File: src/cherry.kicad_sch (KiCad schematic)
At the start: 72 parts, among them J1 USB4085-GF-A, J2 PinHeader_1x24, J3 PinHeader_1x06, J4 PinHeader_1x06, J5 PinHeader_1x06, J6 PinHeader_1x24, SW1 RESET, SW2 USER, U1 FT2232HQ, U2 ICE40LP8K-CM81, U3 W25Q32JVSSIQ, U4 TPS62A02, U5 TPS62A02, X1 ASE-12.000MHZ-LC-T

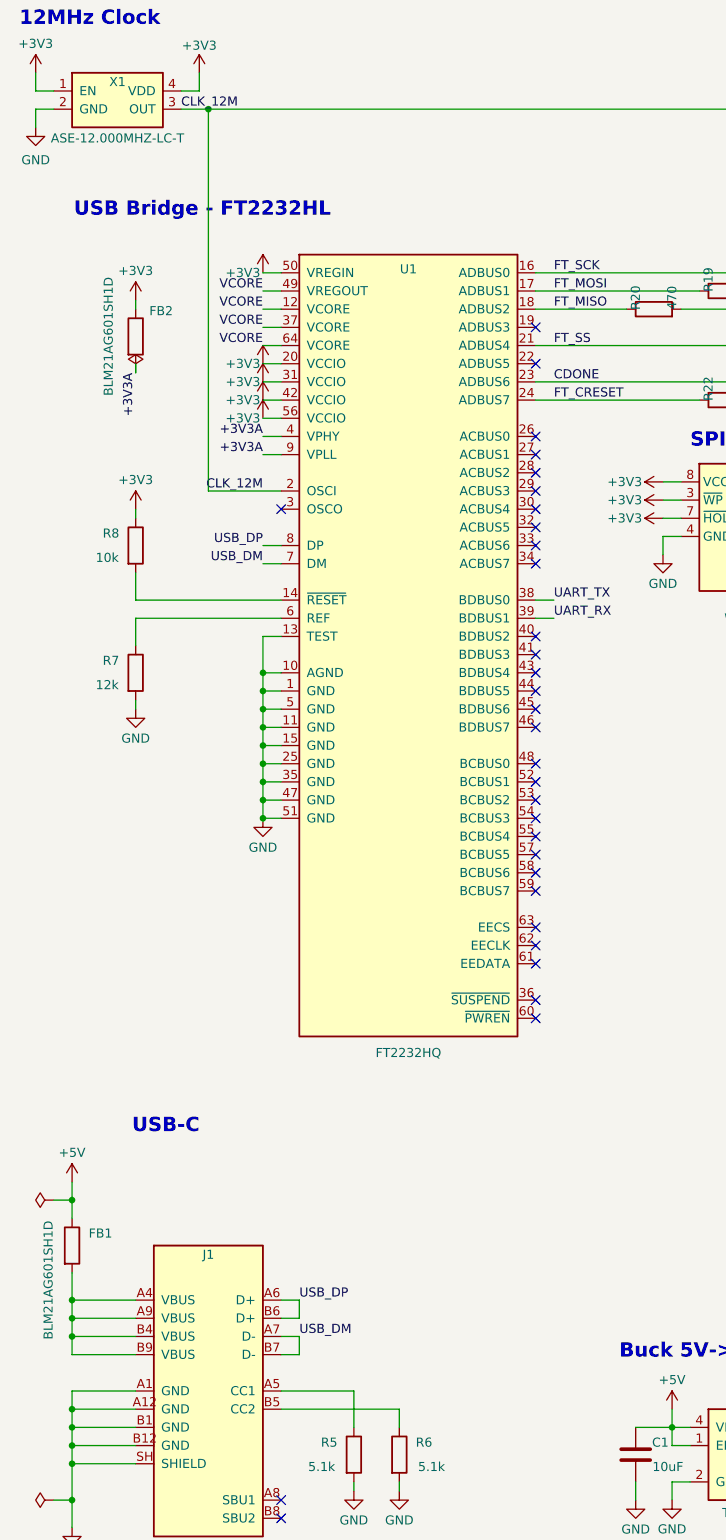
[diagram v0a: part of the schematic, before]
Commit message: 56Q
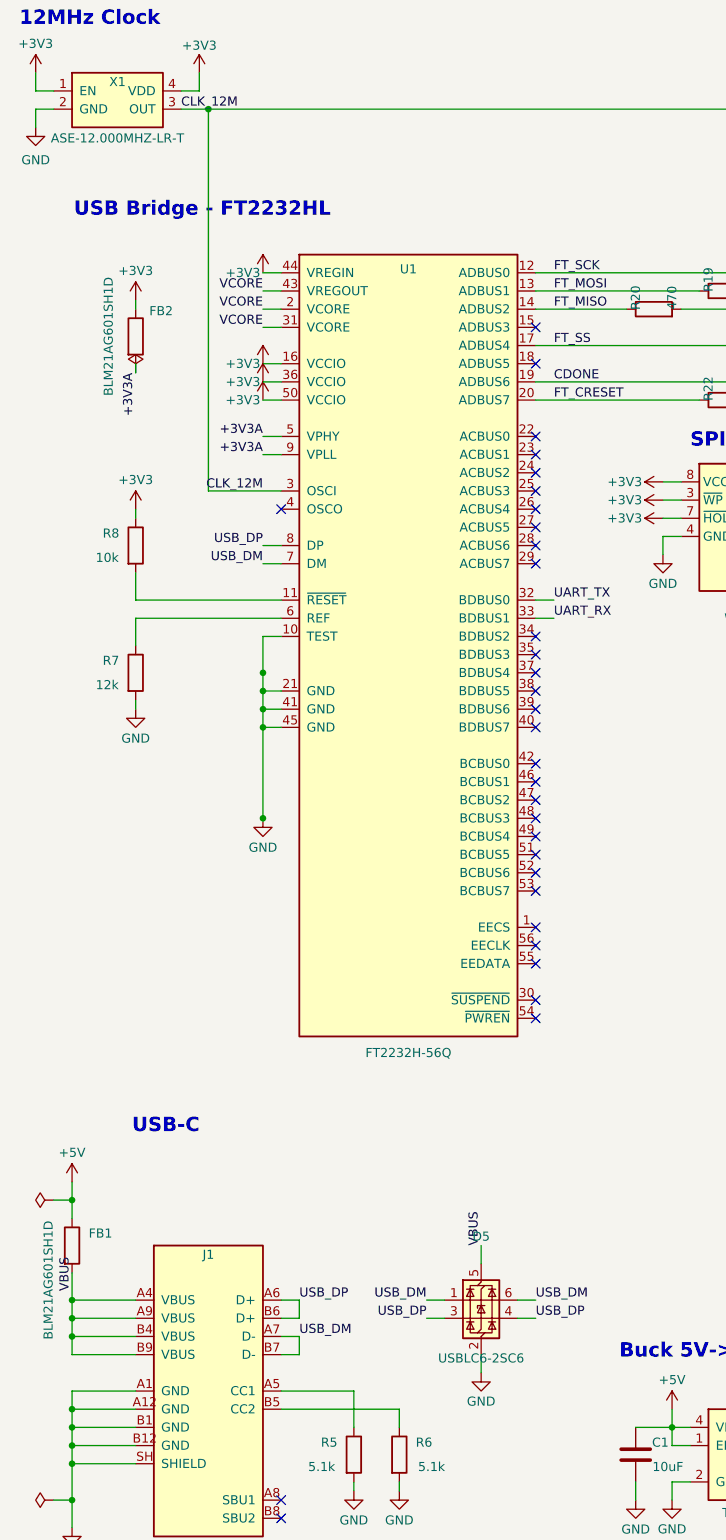
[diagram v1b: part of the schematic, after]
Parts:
- added D5: USBLC6-2SC6, Cherry:SOT-23-6, symbol Cherry:USBLC6-2SC6
- U1: value FT2232HQ -> FT2232H-56Q; footprint Cherry:QFN-64-1EP_9x9mm_P0.5mm_EP4.35x4.35mm -> Cherry:QFN-56-1EP_8x8mm_P0.5mm_EP5.9x5.9mm; symbol Cherry:FT2232HL -> Cherry:FT2232H-56Q
- U3: footprint Cherry:SOIC-8_3.9x4.9mm_P1.27mm -> Cherry:SOIC-8_5.3x5.3mm_P1.27mm
- X1: value ASE-12.000MHZ-LC-T -> ASE-12.000MHZ-LR-T
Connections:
- net +3V3: now also U1.16 (VCCIO), U1.36 (VCCIO), U1.44 (VREGIN); no longer U1.20 (VCCIO), U1.31 (VCCIO), U1.42 (VCCIO), U1.56 (VCCIO)
- net +3V3A: now also U1.5 (VPHY); no longer U1.4 (VPHY)
- net CDONE: now also U1.19 (ADBUS6); no longer U1.23 (ADBUS6)
- net CLK_12M: now also U1.3 (OSCI); no longer U1.2 (OSCI)
- net FT_CRESET: now also U1.20 (ADBUS7); no longer U1.24 (ADBUS7)
- net FT_MISO: now also U1.14 (ADBUS2); no longer U1.18 (ADBUS2)
- net FT_MOSI: now also U1.13 (ADBUS1); no longer U1.17 (ADBUS1)
- net FT_SCK: now also U1.12 (ADBUS0); no longer U1.16 (ADBUS0)
- net FT_SS: now also U1.17 (ADBUS4); no longer U1.21 (ADBUS4)
- net GND: now also U1.21 (GND), U1.41 (GND), U1.45 (GND), U1.57 (GND), D5.2 (GND); no longer U1.1 (GND), U1.11 (GND), U1.13 (TEST), U1.15 (GND), U1.25 (GND), U1.35 (GND), U1.47 (GND), U1.5 (GND), U1.51 (GND), U1.65 (GND)
- net UART_RX: now also U1.33 (BDBUS1); no longer U1.39 (BDBUS1)
- net UART_TX: now also U1.32 (BDBUS0); no longer U1.38 (BDBUS0)
- net USB_DM: now also D5.1 (I/O1), D5.6 (I/O1)
- net USB_DP: now also D5.3 (I/O2), D5.4 (I/O2)
- net VCORE: now also U1.2 (VCORE), U1.31 (VCORE), U1.43 (VREGOUT); no longer U1.12 (VCORE), U1.37 (VCORE), U1.49 (VREGOUT), U1.64 (VCORE)
- net at R8.2: now also U1.11 (~{RESET}); no longer U1.14 (~{RESET})
- net VBUS: now reaches FB1.2, J1.A4 (VBUS), J1.A9 (VBUS), J1.B4 (VBUS), J1.B9 (VBUS)
- net VBUS: now also D5.5 (VBUS)
